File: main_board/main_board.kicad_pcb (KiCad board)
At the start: 2 copper layers, 145 x 91 mm, 132 parts, among them J1 stepper 0, J10 24VDC output 5, J11 5VDC output 0, J12 5VDC output 1, J13 5VDC output 2, J14 5VDC output 3, J15 5VDC output 4, J16 5VDC output 5, J17 temperature measure 0, J18 temperature measure 1, J19 I2C, J2 stepper 1, J20 I2C, J21 I2C, J22 I2C, J23 hall measure 0, J24 weight measure 0, J25 light measure 0, J26 24VDC_in, J27 24VDC to 5VDC step down, J28 24VDC, J29 24VDC, J3 stepper 2, J30 24VDC, J31 5VDC, J32 5VDC, J33 5VDC, J34 hall measure 1, J35 reflective sensor 0, J36 24VDC, J37 24VDC, J38 24VDC, J39 5VDC, J4 stepper 3, J40 5VDC, J41 5VDC, J42 Conn_01x05_Male, J5 24VDC output 0, J6 24VDC output 1, J7 24VDC output 2, J8 24VDC output 3, J9 24VDC output 4, Q1 Q_NMOS_GDS, Q10 BS170, Q11 BS170, Q12 BS170, Q2 Q_NMOS_GDS, Q3 Q_NMOS_GDS, Q4 Q_NMOS_GDS, Q5 Q_NMOS_GDS, Q6 Q_NMOS_GDS, Q7 BS170, Q8 BS170, Q9 BS170, U1 ESP32-DEVKITC-32D, U2 PCA9685PW

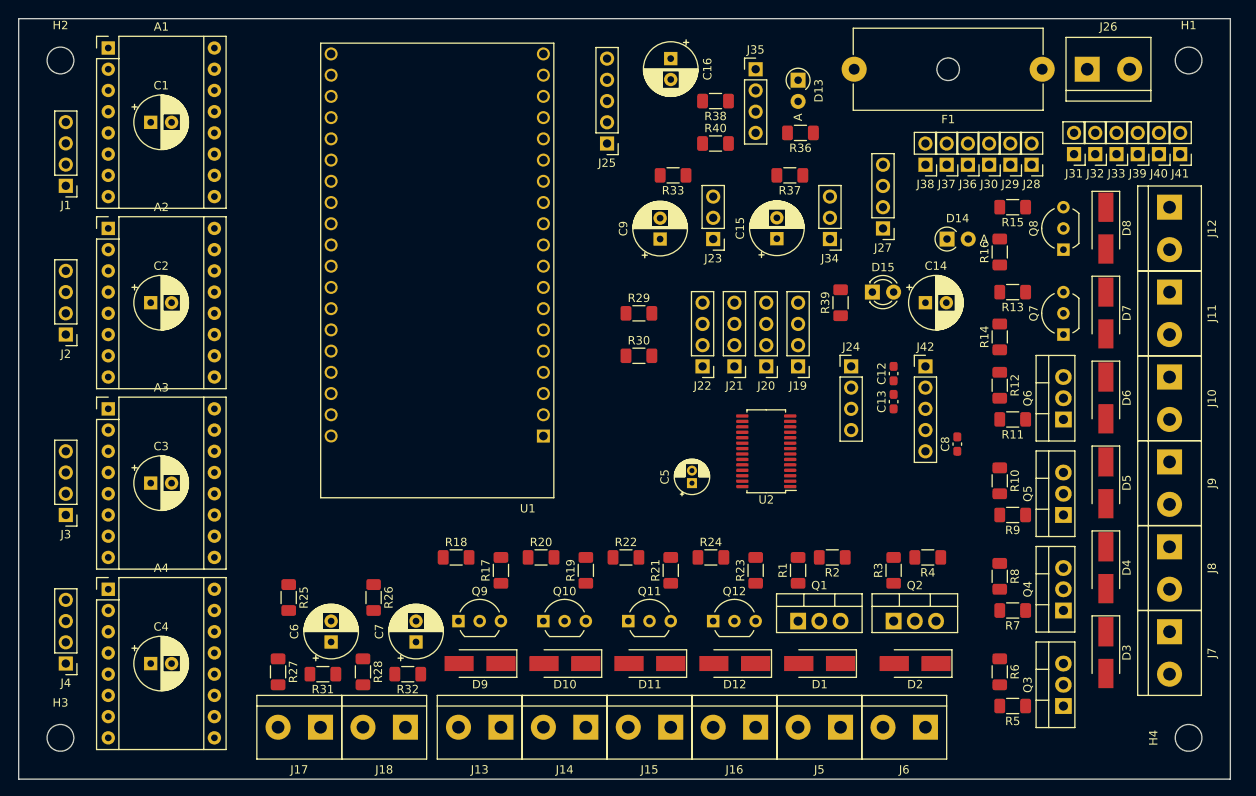
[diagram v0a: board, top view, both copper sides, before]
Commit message: added routs
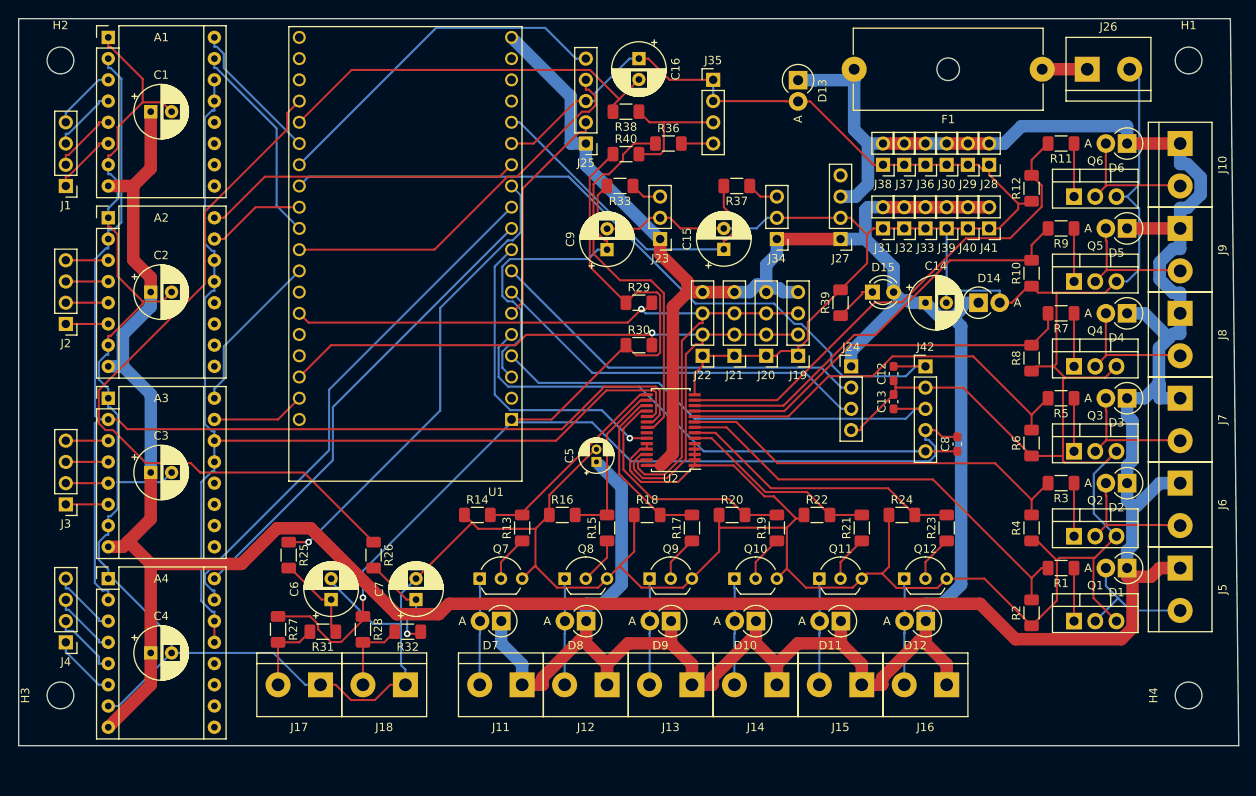
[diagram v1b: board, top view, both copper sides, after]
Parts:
- D1, D10, D11, D12, D2, D3, D4, D5, D6, D7, D8, D9: footprint Diode_SMD:D_SMA_Handsoldering -> Diode_THT:D_DO-15_P2.54mm_Vertical_AnodeUp
- D13, D14: footprint Diode_THT:D_A-405_P2.54mm_Vertical_AnodeUp -> Diode_THT:D_DO-15_P2.54mm_Vertical_AnodeUp
- moved J11 90.6 mm to (95.2, 92.7), turned to 180 degrees
- moved J12 88.3 mm to (105.4, 92.7), turned to 180 degrees
- moved D7 81.2 mm to (92.8, 85.1), turned to 180 degrees
- moved D8 78.0 mm to (102.9, 85.1), turned to 180 degrees
- moved Q7 75.7 mm to (90.2, 80.0), turned to 0 degrees
- moved Q8 71.5 mm to (100.3, 80.0), turned to 0 degrees
- moved R14 66.0 mm to (89.9, 72.4), turned to 0 degrees
- moved R13 65.1 mm to (95.2, 73.9), turned to 90 degrees
- moved R15 61.9 mm to (105.4, 73.9), turned to 90 degrees
- moved R16 61.1 mm to (100.0, 72.4), turned to 0 degrees
- moved J5 44.9 mm to (174.0, 78.7), turned to 270 degrees
- moved J6 42.2 mm to (174.0, 68.6), turned to 270 degrees
- moved D1 38.5 mm to (167.6, 78.7)
- moved R5 37.3 mm to (159.7, 58.4)
- moved R7 36.0 mm to (159.7, 48.3)
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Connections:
- U2 pad 10: 24VDC_output4 -> 24VDC_output2
- U2 pad 11: 24VDC_output5 -> 24VDC_output3
- U2 pad 12: 5VDC_output0 -> 24VDC_output4
- U2 pad 13: 5VDC_output1 -> 24VDC_output5
- U2 pad 15: 5VDC_output2 -> 5VDC_output0
- U2 pad 16: 5VDC_output3 -> 5VDC_output1
- U2 pad 17: 5VDC_output4 -> 5VDC_output2
- U2 pad 18: 5VDC_output5 -> 5VDC_output3
- U2 pad 6: 24VDC_output0 -> 5VDC_output4
- U2 pad 7: 24VDC_output1 -> 5VDC_output5
- U2 pad 8: 24VDC_output2 -> 24VDC_output0
- U2 pad 9: 24VDC_output3 -> 24VDC_output1
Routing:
- net GND: track 0.00 -> 676.5 mm
- net +24V: track 0.00 -> 381.4 mm
- net +5V: track 0.00 -> 307.5 mm
- net +3V3: track 0.00 -> 159.5 mm, vias 0 -> 1
- net stepperErr: track 0.00 -> 143.7 mm
- net stepperON: track 0.00 -> 130.7 mm
- net enca: track 0.00 -> 90.3 mm
- net SCL: track 0.00 -> 90.0 mm, vias 0 -> 1
- net SDA: track 0.00 -> 89.3 mm, vias 0 -> 1
- net Net-(R26-Pad1): track 0.00 -> 87.3 mm
- net button: track 0.00 -> 64.3 mm
- net STEP3: track 0.00 -> 62.8 mm
- net 24VDC_output5: track 0.00 -> 60.0 mm
- net encb: track 0.00 -> 57.0 mm
- net DIR3: track 0.00 -> 56.6 mm
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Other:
- board size 145 x 91 mm -> 146 x 87 mm
